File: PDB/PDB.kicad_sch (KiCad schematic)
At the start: 33 parts

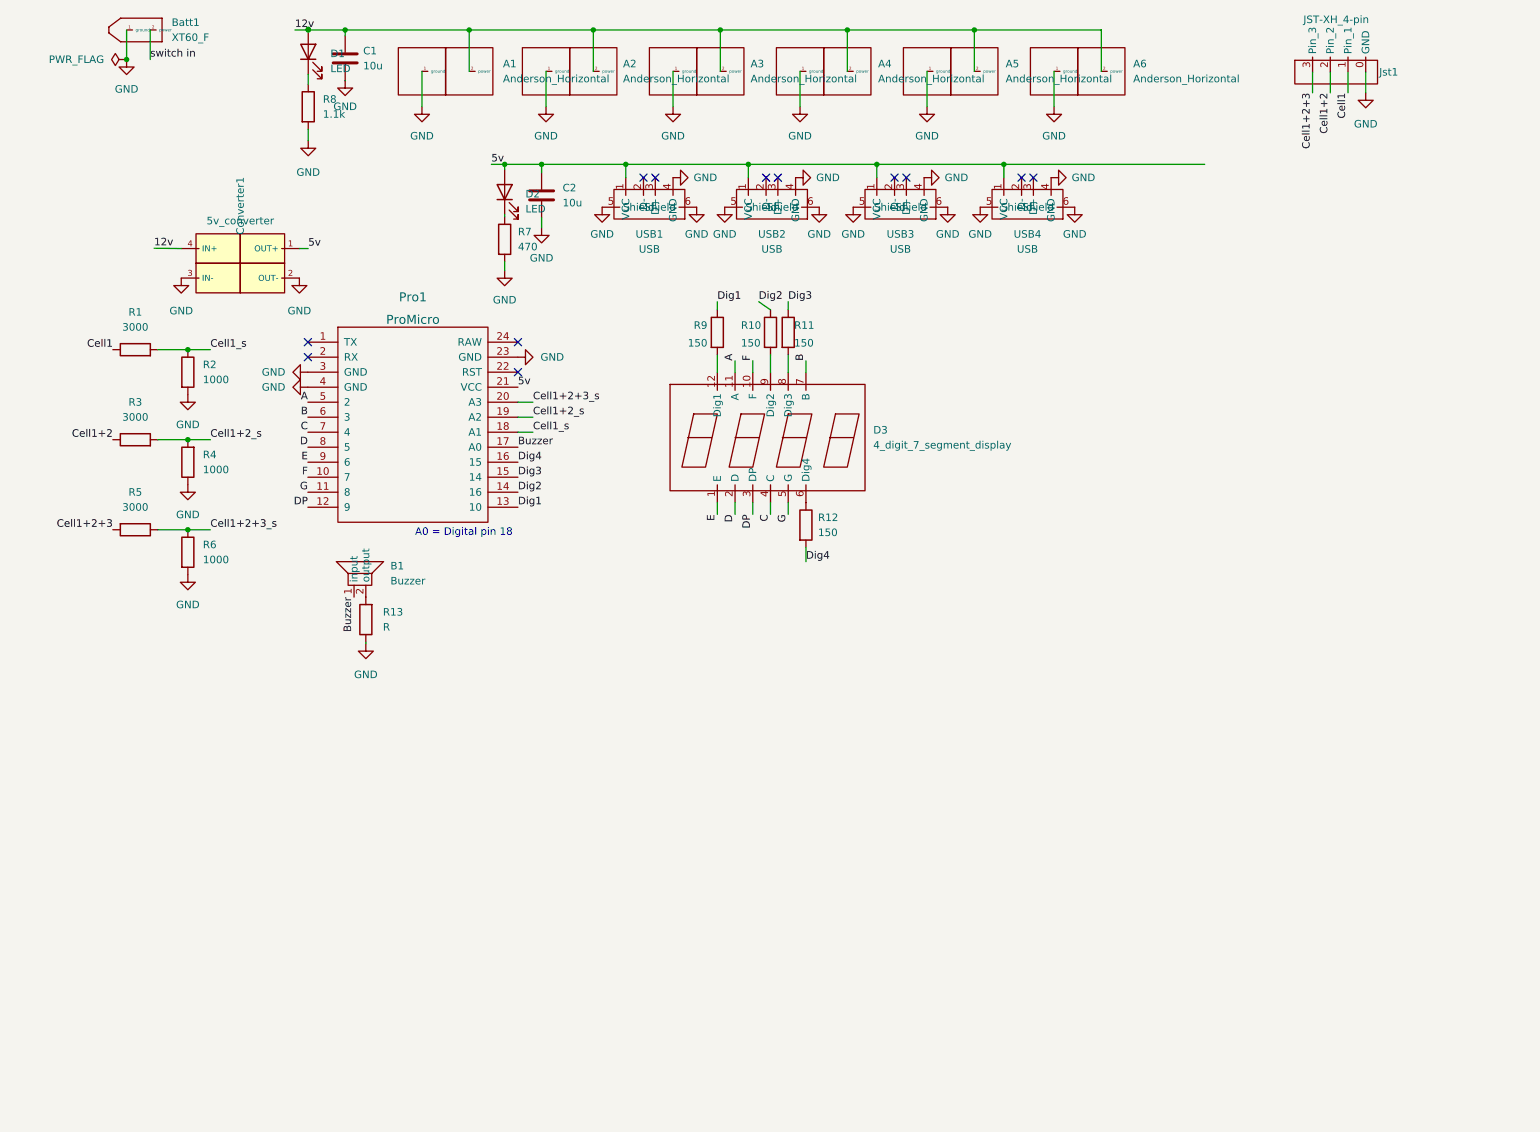
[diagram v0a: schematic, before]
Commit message: finished Schematic
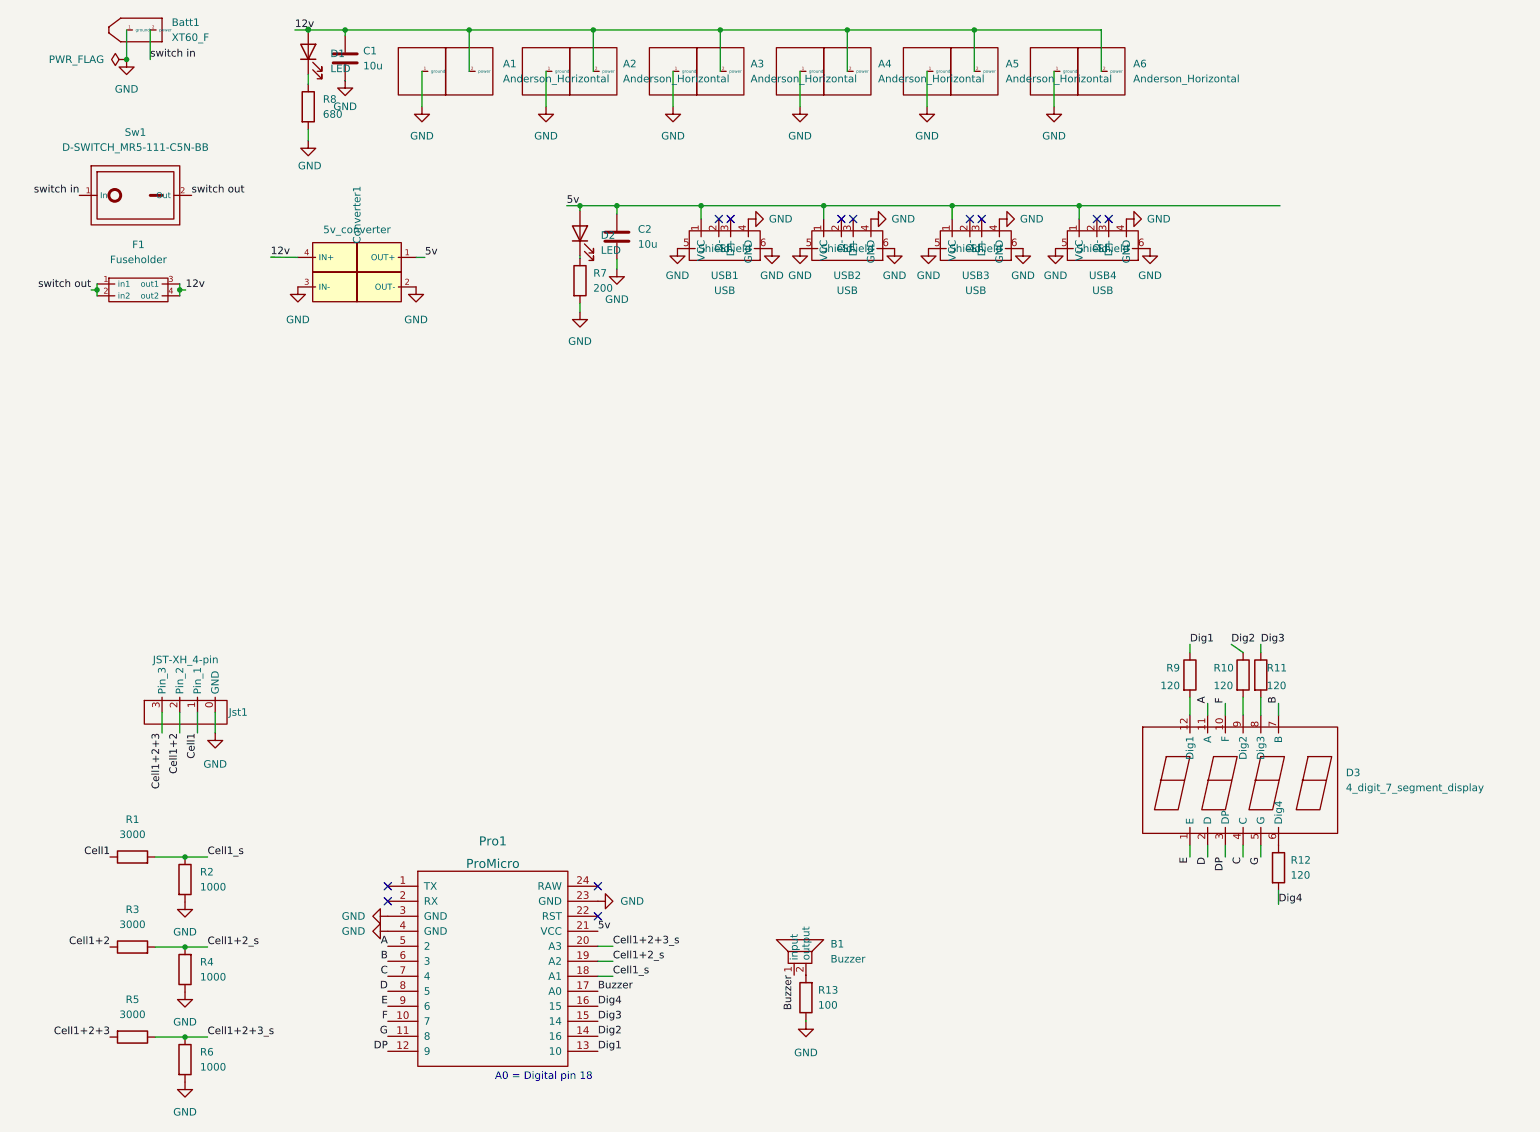
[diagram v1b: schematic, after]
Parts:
- added F1: Fuseholder, symbol PiE_Symbols:Fuseholder
- added Sw1: D-SWITCH_MR5-111-C5N-BB, symbol PiE_Symbols:D-SWITCH_MR5-111-C5N-BB
- R10, R11, R12, R9: value 150 -> 120
- R13: value R -> 100
- R7: value 470 -> 200
- R8: value 1.1k -> 680
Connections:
- net 12v: now also F1.3 (out1), F1.4 (out2)
- net switch in: now also Sw1.1 (In)
- new net switch out: F1.1 (in1), F1.2 (in2), Sw1.2 (Out)
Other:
- moved on the sheet: B1, C2, Converter1, D2, D3, Jst1, Pro1, R1, R10, R11, R12, R13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
